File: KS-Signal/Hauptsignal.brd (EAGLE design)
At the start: 24.6 x 48 mm, 20 parts, among them IC1 ATTINY44SSU

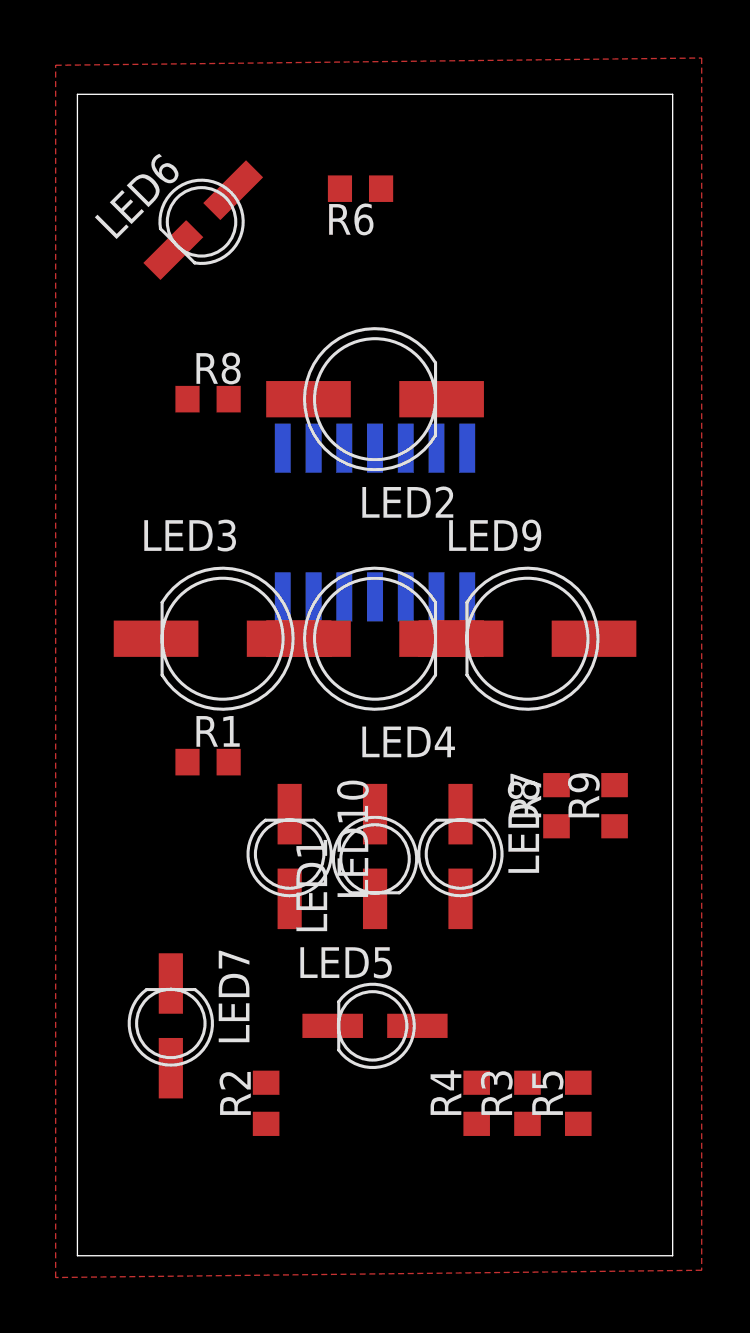
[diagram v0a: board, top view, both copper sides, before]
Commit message: Rückseite fertig
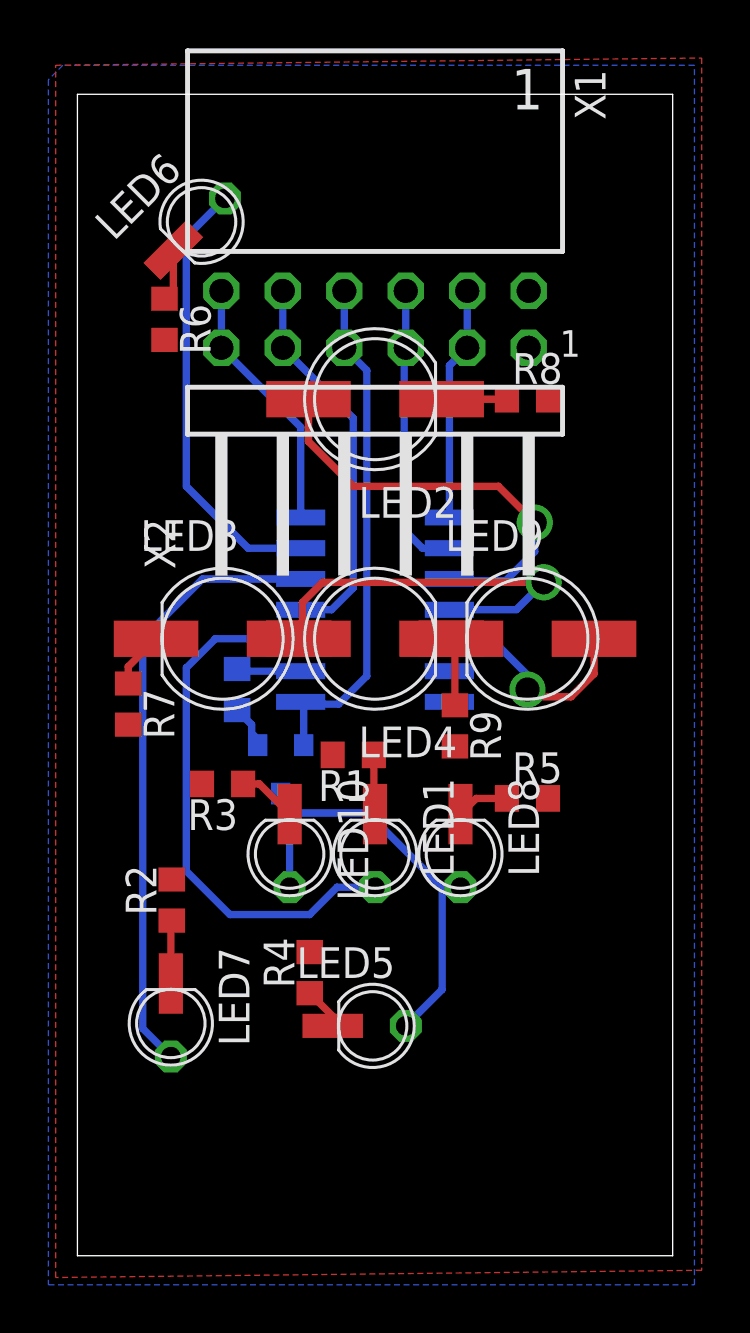
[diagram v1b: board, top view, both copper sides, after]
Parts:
- added Q1: IRLML5203, transistor-power:MICRO3
- added R10: (no value), rcl:R0603
- added X1: SSW-106-02-S-S-RA, con-samtec:SSW-106-02-S-S-RA
- added X2: TSW-106-02-S-S-RA, con-samtec:TSW-106-02-S-S-RA
- LED1, LED10, LED5, LED6, LED7, LED8: value LED_SMD3MM -> LED_SMD3MM_SMD/DIP; device LEDFLATTOP:3MM_FLAT_SMDLED -> LEDFLATTOP:3MM_FLAT/DIP_SMDLED
- LED2, LED3, LED4, LED9: value LED_SMD5MM -> LED_SMD5MM_SMD
- moved R3 18.2 mm to (6.00, 19.5), turned to 180 degrees
- moved R7 18.2 mm to (2.10, 22.8), turned to 270 degrees
- moved R8 13.2 mm to (18.6, 35.4)
- moved R5 12.8 mm to (18.6, 18.9), turned to 0 degrees
- moved R6 9.73 mm to (3.60, 38.7), turned to 270 degrees
- moved R2 9.26 mm to (3.90, 14.7)
- moved R4 8.76 mm to (9.60, 11.7)
- moved R9 7.38 mm to (15.6, 21.9), turned to 270 degrees
- moved R1 6.01 mm to (11.4, 20.7), turned to 180 degrees
- moved IC1 3.60 mm to (12.3, 26.7), turned to 90 degrees
- turned LED1 to 270 degrees
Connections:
- new net MISO: IC1.8, X1.2, X2.2
- new net N$10: LED10.+, LED5.+, LED8.+, Q1.3
- new net N$11: Q1.1, R10.2
- new net RESET: IC1.4, X1.5, X2.5
- new net SCL/SCK: IC1.9, X1.3, X2.3
- new net SDA/MOSI: IC1.7, X1.6, X2.6
- net GE: now also IC1.12
- net GN: now also IC1.11
- net GND: now also X1.1, X2.1
- net N$1: now also LED4.-
- net N$8: no longer LED4.-
- net RT: now also IC1.10
- net SH1: now also IC1.5
- net SH1ZS1: now also IC1.3
- net VCC: now also Q1.2, X1.4, X2.4
- net ZL: now also IC1.6
- net ZS7: now also IC1.2, R10.1; no longer LED10.+, LED5.+, LED8.+
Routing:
- net SH1: track 0.00 -> 25.3 mm
- net SH1ZS1: track 0.00 -> 22.7 mm
- net VCC: track 0.00 -> 21.4 mm
- net N$10: track 0.00 -> 18.8 mm
- net ZL: track 0.00 -> 18.3 mm
- net RT: track 0.00 -> 17.7 mm, vias 0 -> 1
- net GN: track 0.00 -> 16.3 mm, vias 0 -> 1
- net RESET: track 0.00 -> 16.0 mm
- net SCL/SCK: track 0.00 -> 12.1 mm
- net SDA/MOSI: track 0.00 -> 10.7 mm
- net MISO: track 0.00 -> 9.67 mm
- net GE: track 0.00 -> 9.19 mm, vias 0 -> 1
- net N$1: track 0.00 -> 2.85 mm
- net N$9: track 0.00 -> 2.70 mm
- net ZS7: track 0.00 -> 2.66 mm
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- added copper zone on layer 16, net GND
